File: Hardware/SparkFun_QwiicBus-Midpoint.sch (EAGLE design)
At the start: 49 parts, among them J1 QWIIC, J2 QWIIC, J3 RJ45, J7 RJ45, U1 PCA9615, U3 LMR33630

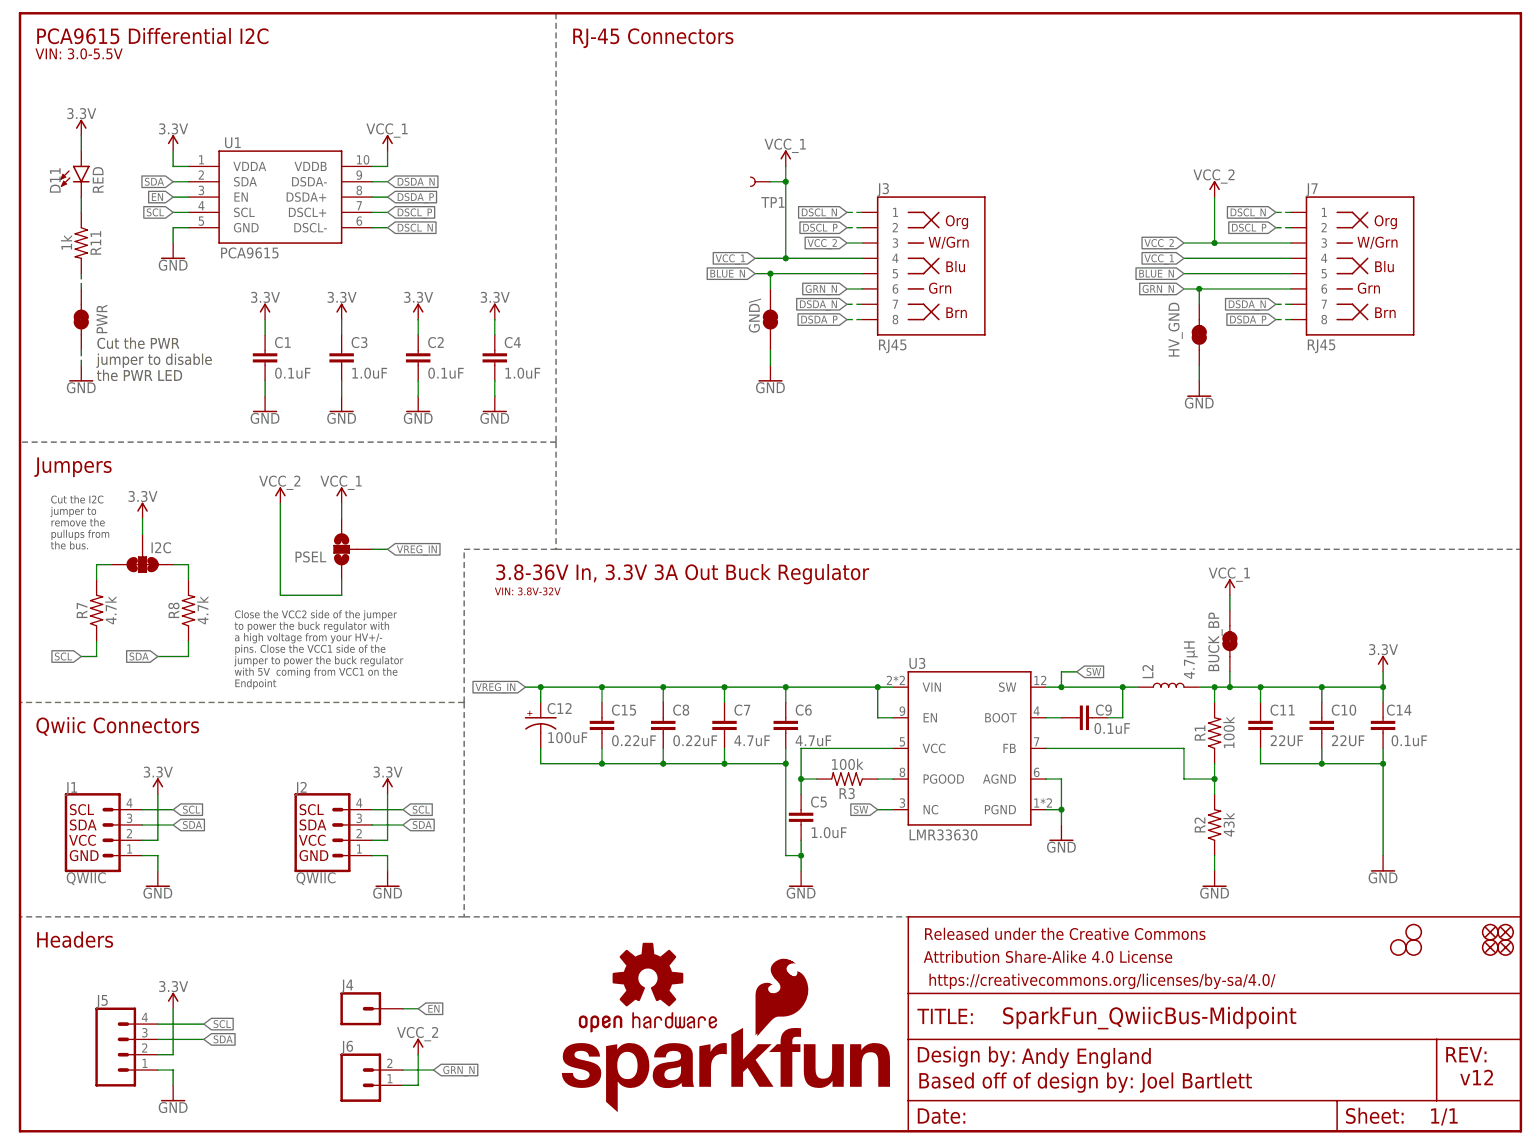
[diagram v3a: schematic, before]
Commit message: post checklist changes
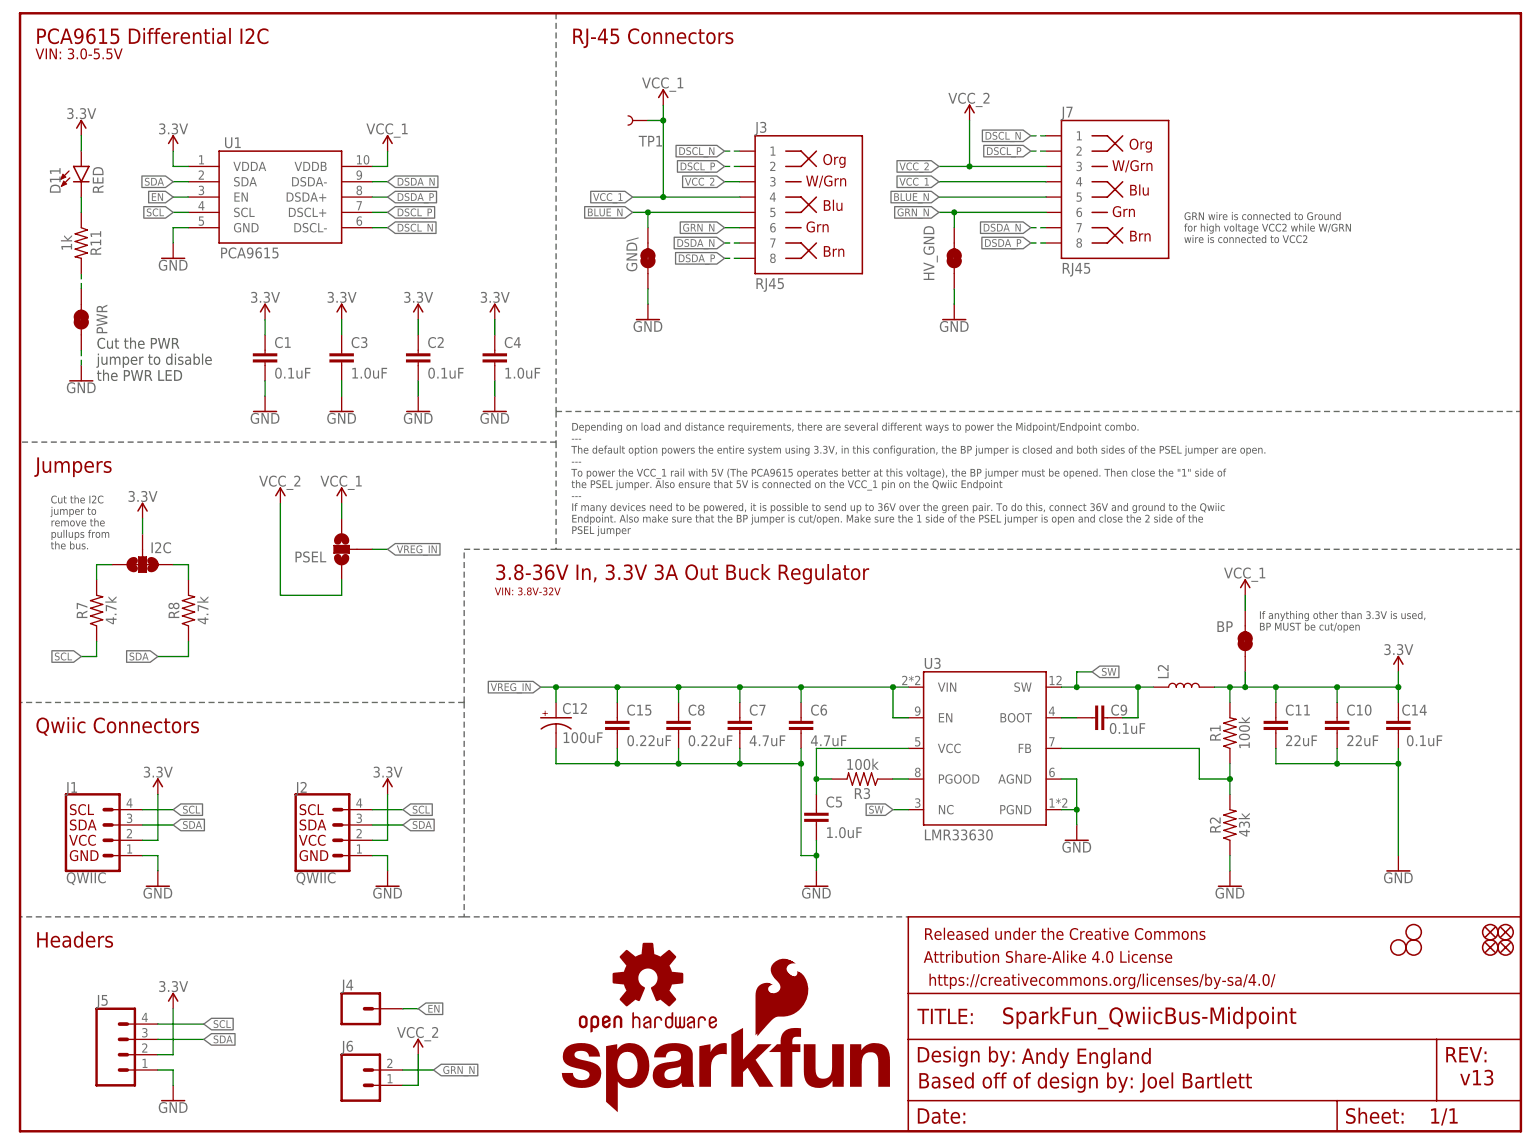
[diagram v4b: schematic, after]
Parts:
- removed BUCK_BP: JUMPER-SMT_2_NC_TRACE_SILK, SparkFun-Jumpers:JUMPER-SMT_2_NC_TRACE_SILK
- added BP: JUMPER-SMT_2_NC_TRACE_SILK, SparkFun-Jumpers:JUMPER-SMT_2_NC_TRACE_SILK
- C10, C11: value 22UF -> 22uF
- C15, C8: device SparkFun-Capacitors:0.22UF-0603-25V-10% -> SparkFun-Capacitors:0.22UF-0603-50V-10%
- L2: value 4.7μH -> 2.2uH; device SparkFun-Coils:4.7μH_SHIELDED_INDUCTORNPIS_LS -> SparkFun-Coils:2.2μH_SHIELDED_INDUCTOR_5X5
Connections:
- net 3.3V: now also BP.1; no longer BUCK_BP.1
- net VCC_1: now also BP.2; no longer BUCK_BP.2
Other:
- note added: "Depending on load and distance requirements, there are several different ways to power the Midpoint/Endpoint combo. --- The default option powers the entire system using 3.3V, in this configuration, the BP jumper is closed and both sides of the PSEL jumper are open. --- To power the VCC_1 rail with 5V (The PCA9615 operates better at this voltage), the BP jumper must be opened. Then close the "1" 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"
- note added: "GRN wire is connected to Ground for high voltage VCC2 while W/GRN wire is connected to VCC2"
- note added: "If anything other than 3.3V is used, BP MUST be cut/open"
- note added: "v13"
- note removed: "Close the VCC2 side of the jumper to power the buck regulator with a high voltage from your HV+/- pins. Close the VCC1 side of the jumper to power the buck regulator with 5V coming from VCC1 on the Endpoint"
- note removed: "v12"
- moved on the sheet: C10, C11, C12, C14, C15, C5, C6, C7, C8, C9, GND\, HV_GND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
